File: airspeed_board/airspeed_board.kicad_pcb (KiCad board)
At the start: 2 copper layers, 6 parts, among them J1 BME280, J2 ADXL345, J3 MPXV5002DP, U1 ESP32-C3_SUPERMINI, U2 XGZP6897D_1, U3 XGZP6897D_2

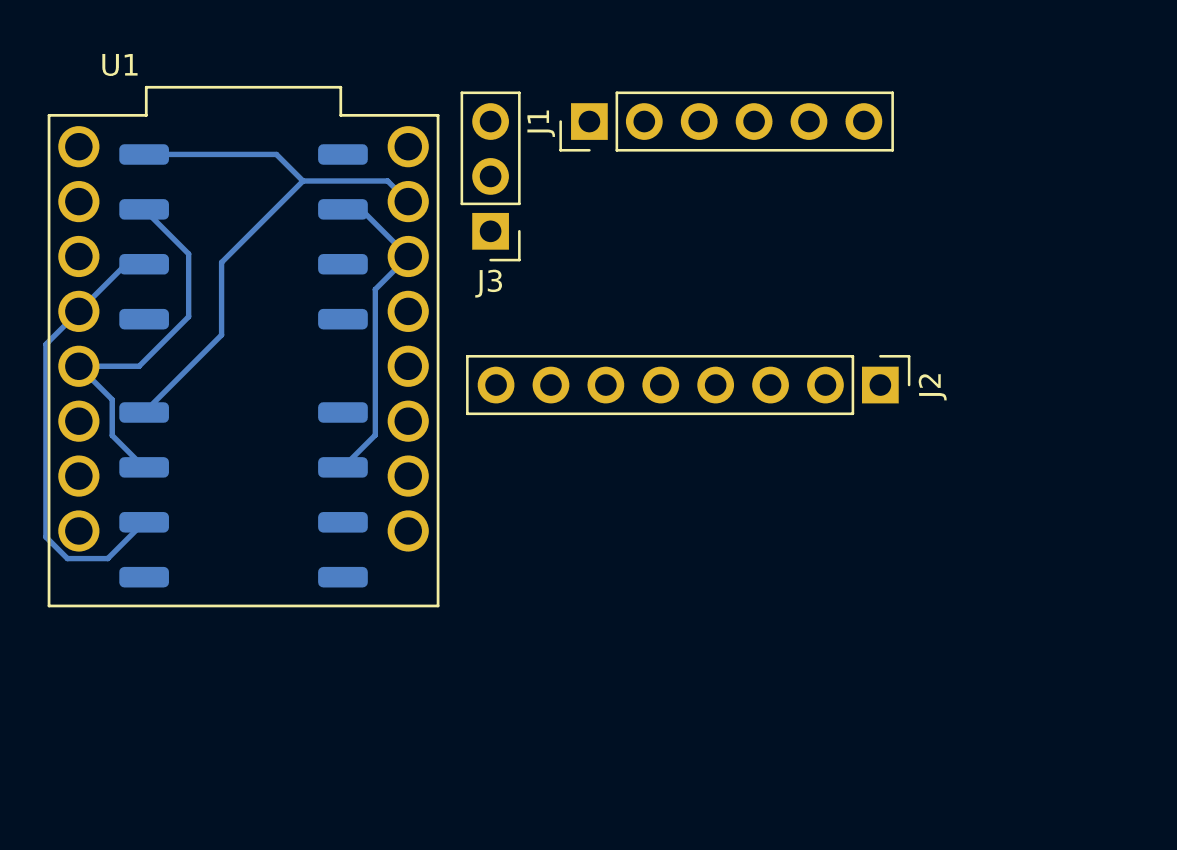
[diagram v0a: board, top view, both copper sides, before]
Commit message: updated board layout
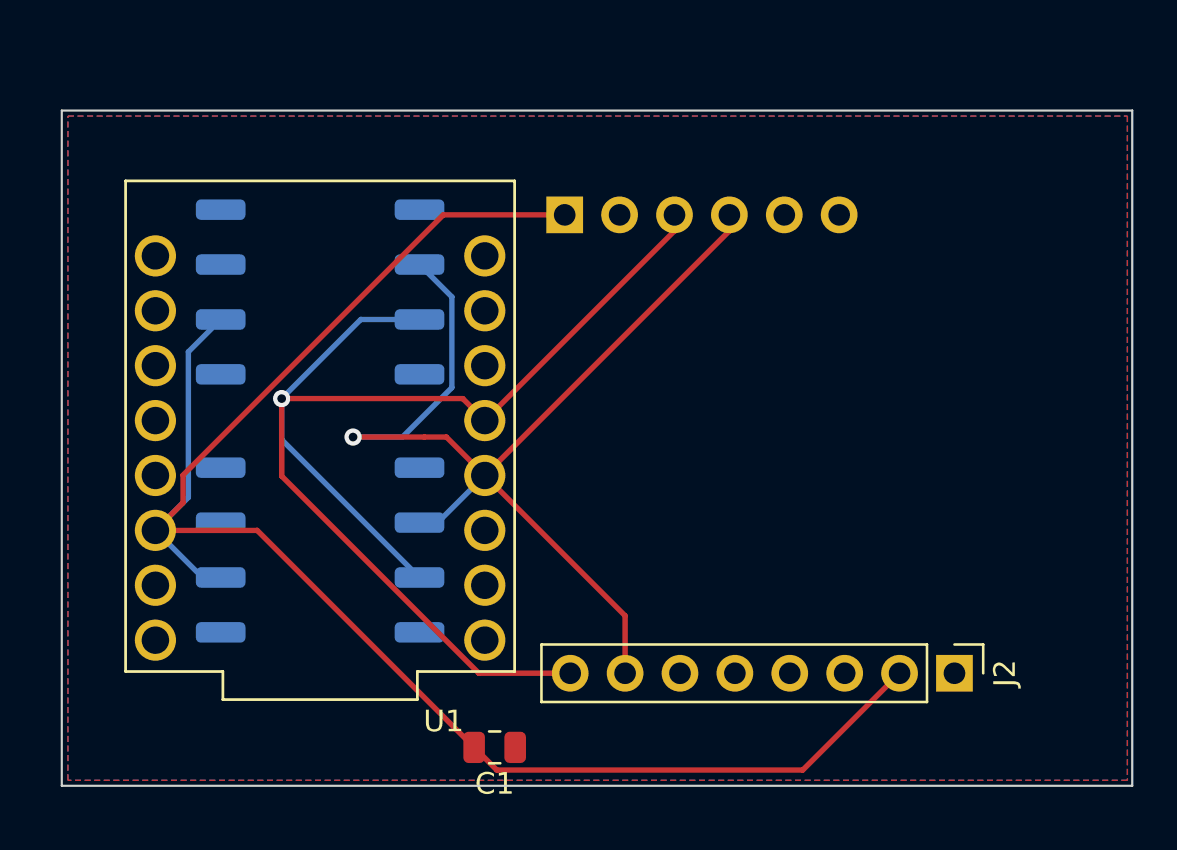
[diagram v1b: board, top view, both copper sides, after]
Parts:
- removed J3: MPXV5002DP, Connector_PinHeader_2.54mm:PinHeader_1x03_P2.54mm_Vertical
- added C1: 0.1uF, Capacitor_SMD:C_0805_2012Metric, F.Cu at (147.0, 80.3)
- J1: moved to B.Cu
- moved U3 14.9 mm to (138.9, 71.1), turned to 0 degrees
- moved J2 13.8 mm to (168.3, 76.8)
- moved U2 10.0 mm to (138.9, 59.2), turned to 0 degrees
- moved U1 4.66 mm to (138.9, 65.4), turned to 180 degrees
- moved J1 4.47 mm to (150.2, 55.6), turned to -90 degrees
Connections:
- J1 pad 1: unconnected-(J1-Pin_1-Pad1) -> 3.3V
- J1 pad 2: unconnected-(J1-Pin_2-Pad2) -> GND
- J1 pad 3: unconnected-(J1-Pin_3-Pad3) -> SCL
- J1 pad 4: unconnected-(J1-Pin_4-Pad4) -> SDA
- J2 pad 1: unconnected-(J2-Pin_1-Pad1) -> GND
- J2 pad 2: unconnected-(J2-Pin_2-Pad2) -> 3.3V
- J2 pad 7: unconnected-(J2-Pin_7-Pad7) -> SDA
- J2 pad 8: unconnected-(J2-Pin_8-Pad8) -> SCL
- U1 pad 5V: unconnected-(U1-Pad5V) -> 5V
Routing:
- net 3.3V: track 14.9 -> 81.5 mm
- net SCL: track 17.8 -> 62.5 mm, vias 0 -> 1
- net SDA: track 20.6 -> 51.2 mm, vias 0 -> 1
- net GND: track 26.9 -> 0.00 mm
- added copper zone on B.Cu, net GND
- added copper zone on F.Cu, net GND
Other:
- board outline added: 49.5 x 31.2 mm
